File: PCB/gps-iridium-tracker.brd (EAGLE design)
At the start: 35 x 49.3 mm, 67 parts, among them J1 MICRO-USB, U1 ATMEGA32U4-XUMU, U2 LMR62421, U3 MCP73831

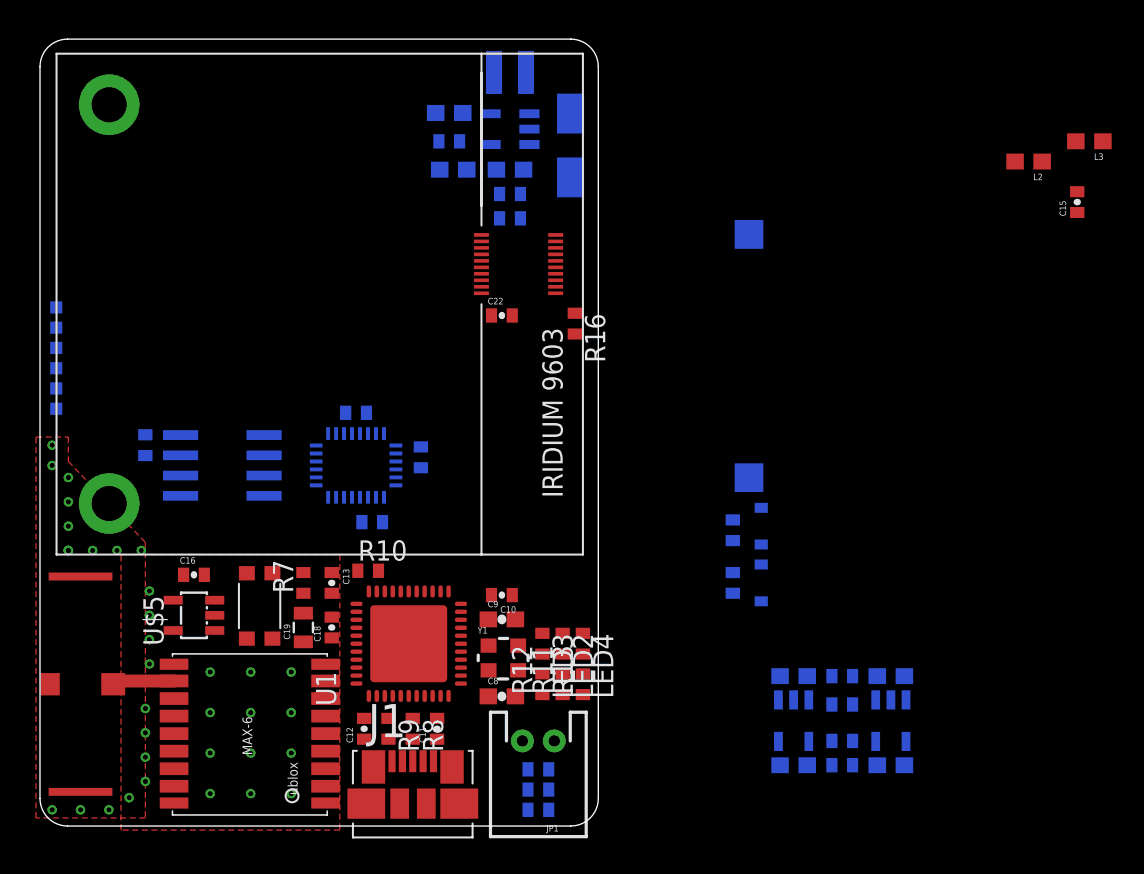
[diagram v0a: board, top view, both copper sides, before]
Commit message: PCB
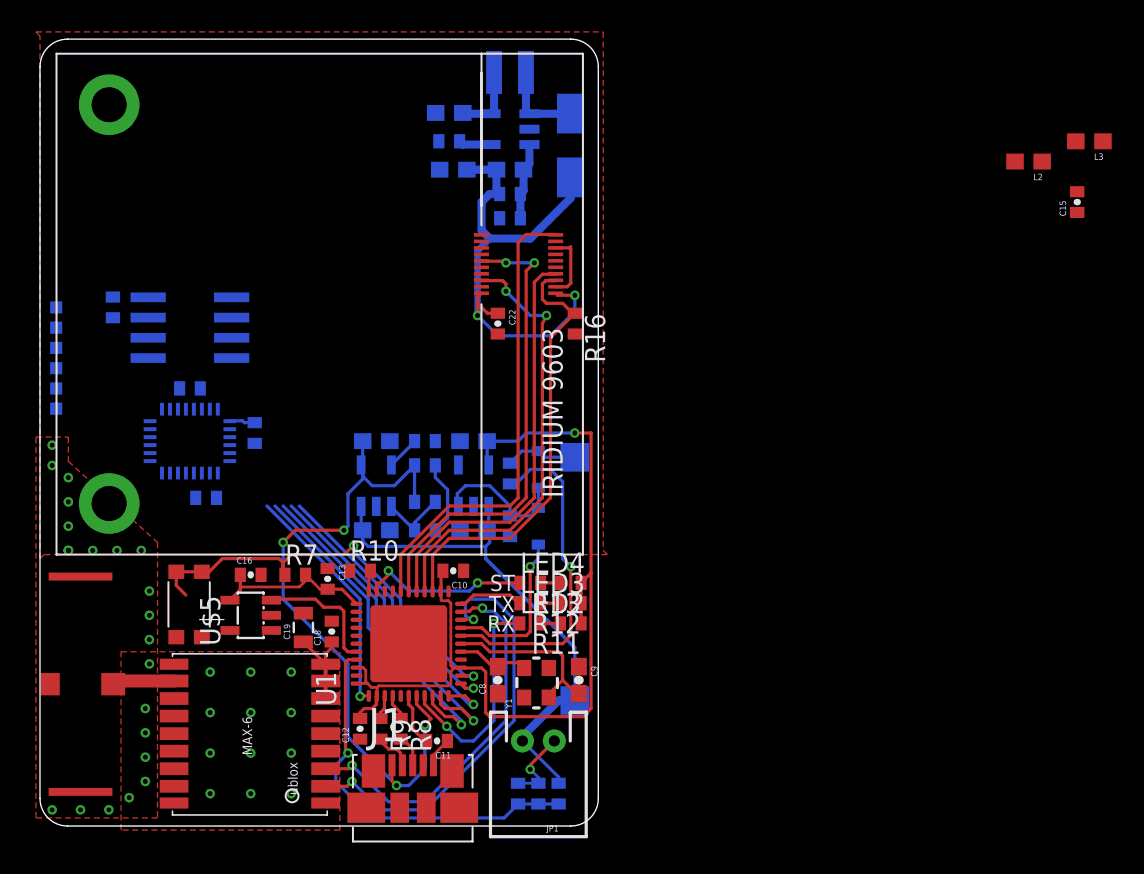
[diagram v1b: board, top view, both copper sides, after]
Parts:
- Y1: value (none) -> 8Z
- moved C4 38.1 mm to (21.1, 24.1), turned to 0 degrees
- moved U3 35.5 mm to (21.1, 21.3), turned to 0 degrees
- moved C5 33.5 mm to (21.1, 18.5), turned to 180 degrees
- moved R6 33.1 mm to (24.1, 24.1), turned to 0 degrees
- moved LED1 31.3 mm to (24.1, 22.6), turned to 0 degrees
- moved R5 29.1 mm to (24.1, 20.3), turned to 180 degrees
- moved C7 28.6 mm to (27.2, 24.1), turned to 0 degrees
- moved R4 27.7 mm to (24.1, 18.5), turned to 0 degrees
- moved U$7 24.9 mm to (27.2, 21.3), turned to 0 degrees
- moved C6 22.1 mm to (27.2, 18.5), turned to 180 degrees
- moved SW1 17.7 mm to (33.5, 15.5), turned to 90 degrees
- moved D2 14.4 mm to (31.2, 22.4)
- moved D3 14.4 mm to (31.2, 18.8)
- moved R17 14.4 mm to (29.5, 18.8)
- moved R18 14.4 mm to (29.5, 22.1)
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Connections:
- net GND: now also Y1.2, Y1.4
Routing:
- net 3.3V: track 0.00 -> 75.3 mm, vias 0 -> 1
- net VUSB: track 0.00 -> 43.6 mm, vias 0 -> 4
- net VBAT: track 0.00 -> 37.3 mm
- net 5V: track 0.00 -> 32.4 mm, vias 0 -> 2
- net SAT_AVAIL: track 0.00 -> 29.7 mm
- net SAT_RI: track 0.00 -> 29.5 mm, vias 0 -> 2
- net SAT_TX: track 0.00 -> 27.9 mm, vias 0 -> 2
- net SAT_EN: track 0.00 -> 27.7 mm
- net GPSTX: track 0.00 -> 27.2 mm, vias 0 -> 2
- net RESET: track 0.00 -> 26.9 mm, vias 0 -> 2
- net SAT_RX: track 0.00 -> 26.2 mm
- net GPSRX: track 0.00 -> 23.9 mm, vias 0 -> 2
- net BATT_READ: track 0.00 -> 23.9 mm, vias 0 -> 1
- net MOSI: track 0.00 -> 21.4 mm, vias 0 -> 1
- net SCK: track 0.00 -> 21.4 mm, vias 0 -> 1
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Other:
- board text added: "RX"
- board text added: "ST"
- board text added: "TX"

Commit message: Finished PCB
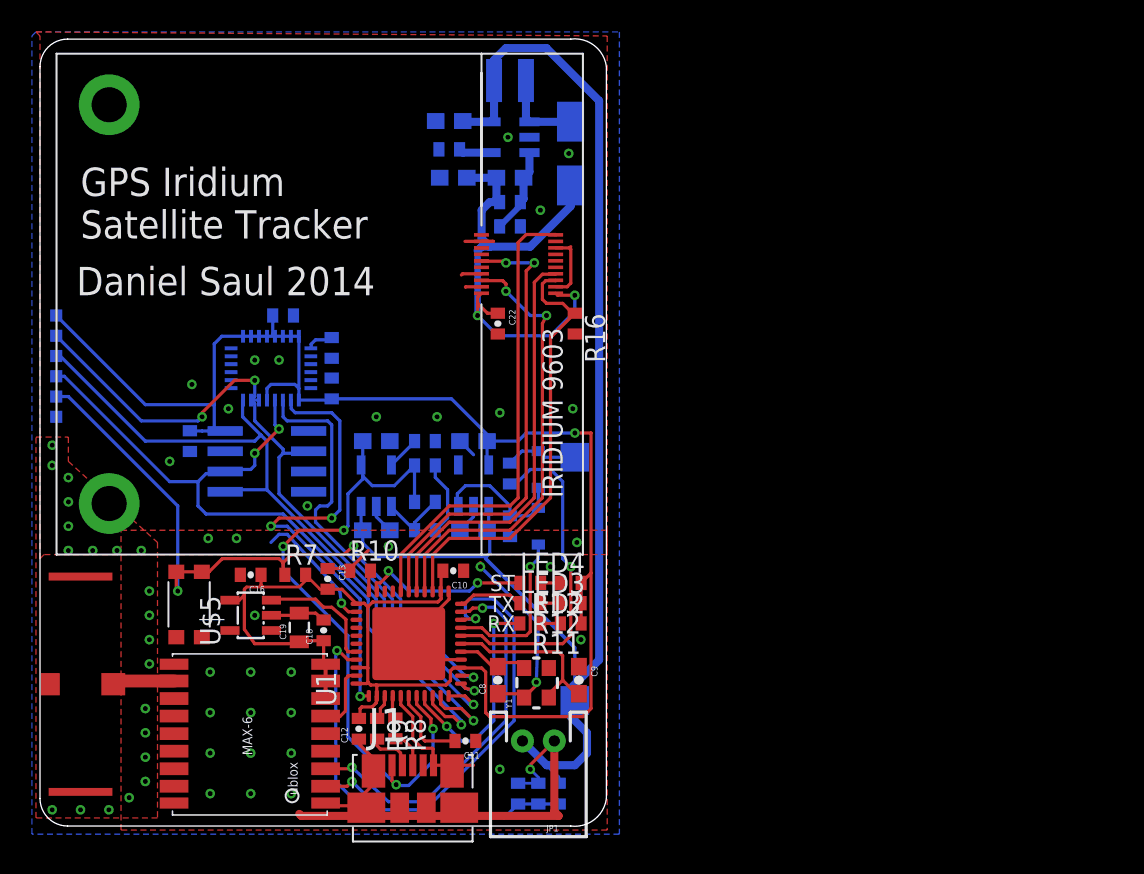
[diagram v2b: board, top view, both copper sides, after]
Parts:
- removed C15: 1pF, apex:0402-CAP
- removed L2, L3: (no value), SparkFun-Passives:0603
- U1: value ATMEGA32U4-XUMU -> SMARTPRJ_ATMEGA32U4-XUMU; device SmartPrj:QFN44ML7X7 -> gps-iridium-tracker:SMARTPRJ_QFN44ML7X7
- moved C17 10.4 mm to (18.3, 27.4), turned to 270 degrees
- moved U$8 9.67 mm to (14.2, 22.9)
- moved C23 9.67 mm to (9.40, 24.1)
- moved C21 7.42 mm to (15.2, 32.0), turned to 0 degrees
- moved C20 7.19 mm to (18.3, 30.0)
- moved U$3 6.83 mm to (14.5, 28.7)
- moved C11 1.78 mm to (26.7, 5.33)
- moved C18 0.51 mm to (17.8, 12.3)
- moved C1 0.51 mm to (25.7, 44.2)
- moved C2 0.51 mm to (25.9, 40.6)
- moved C3 0.51 mm to (29.5, 40.6)
- moved L1 0.51 mm to (29.5, 46.7)
- moved R1 0.51 mm to (29.5, 39.1)
- moved R2 0.51 mm to (29.5, 37.6), turned to 0 degrees
- moved R3 0.51 mm to (25.7, 42.4)
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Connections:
- net 3.3V: now also JP2.P$1; no longer JP2.P$2
- net MISO: now also JP2.P$2; no longer JP2.P$1
- net MOSI: now also JP2.P$3; no longer JP2.P$4
- net SCK: now also JP2.P$4; no longer JP2.P$3
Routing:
- net GND: track 10.9 -> 94.4 mm, vias 35 -> 58
- net 3.3V: track 75.3 -> 132.7 mm
- net VBAT: track 37.3 -> 90.3 mm
- net MISO: track 19.1 -> 46.3 mm, vias 1 -> 3
- net SCK: track 21.4 -> 48.2 mm, vias 1 -> 3
- net MOSI: track 21.4 -> 47.0 mm
- net RESET: track 26.9 -> 42.3 mm, vias 2 -> 3
- net CS_G: track 14.9 -> 28.4 mm, vias 1 -> 3
- net CS_A: track 17.2 -> 27.0 mm
- net N$10: track 3.35 -> 5.13 mm
- net BATT_READ: track 23.9 -> 25.0 mm
- net N$11: track 2.51 -> 3.23 mm
- net N$4: track 4.86 -> 5.40 mm
- added copper zone on layer 16, net GND
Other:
- board size 35 x 49.3 mm -> 35.5 x 49.4 mm
- board text added: "Daniel Saul 2014"
- board text added: "GPS Iridium Satellite Tracker"

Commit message: Changed led resistor values
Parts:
- LED2: value GREEN -> ORANGE
- R11, R12, R13: value 1K -> 47R
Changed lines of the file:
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@@
 <?xml version="1.0" encoding="utf-8"?>
 <!DOCTYPE eagle SYSTEM "eagle.dtd">
-<eagle version="6.3">
+<eagle version="6.4">
 <drawing>
 <settings>
@@
 <setting verticaltext="up"/>
 </settings>
-<grid distance="0.01" unitdist="inch" unit="inch" style="dots" multiple="1" display="yes" altdistance="0.001" altunitdist="inch" altunit="inch"/>
+<grid distance="0.05" unitdist="inch" unit="inch" style="dots" multiple="1" display="yes" altdistance="0.005" altunitdist="inch" altunit="inch"/>
 <layers>
 <layer number="1" name="Top" color="4" fill="1" visible="yes" active="yes"/>
@@
 <layer number="50" name="dxf" color="7" fill="1" visible="no" active="no"/>
 <layer number="51" name="tDocu" color="6" fill="1" visible="yes" active="yes"/>
-<layer number="52" name="bDocu" color="7" fill="1" visible="yes" active="yes"/>
+<layer number="52" name="bDocu" color="7" fill="1" visible="no" active="yes"/>
 <layer number="53" name="tGND_GNDA" color="7" fill="9" visible="no" active="no"/>
 <layer number="54" name="bGND_GNDA" color="1" fill="9" visible="no" active="no"/>
@@
 <element name="C13" library="SparkFun-Passives" package="0402-CAP" value="100nF" x="18.034" y="15.494" rot="R270"/>
 <element name="R10" library="apex" package="R0402" value="10K" x="20.066" y="16.002"/>
-<element name="LED2" library="apex" package="R0402" value="GREEN" x="30.734" y="12.7"/>
+<element name="LED2" library="apex" package="R0402" value="ORANGE" x="30.734" y="12.7"/>
 <element name="LED3" library="apex" package="R0402" value="YELLOW" x="30.734" y="13.97"/>
-<element name="R11" library="apex" package="R0402" value="1K" x="33.274" y="12.7" rot="R180"/>
-<element name="R12" library="apex" package="R0402" value="1K" x="33.274" y="13.97" rot="R180"/>
-<element name="R13" library="apex" package="R0402" value="1K" x="33.274" y="15.24" rot="R180"/>
+<element name="R11" library="apex" package="R0402" value="47R" x="33.274" y="12.7" rot="R180"/>
+<element name="R12" library="apex" package="R0402" value="47R" x="33.274" y="13.97" rot="R180"/>
+<element name="R13" library="apex" package="R0402" value="47R" x="33.274" y="15.24" rot="R180"/>
 <element name="LED4" library="apex" package="R0402" value="RED" x="30.734" y="15.24"/>
 <element name="JP2" library="apex" package="ICSPSMD" value="AVR-ISP-6SMD" x="1.016" y="30.734" rot="MR270"/>
@@
 </signal>
 </signals>
-<errors>
-</errors>
 </board>
 </drawing>
